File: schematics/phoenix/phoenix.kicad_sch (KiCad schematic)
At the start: 11 parts, among them U1 MAX31856, U2 NHD-C0220BIZ, U3 HHG1D-1

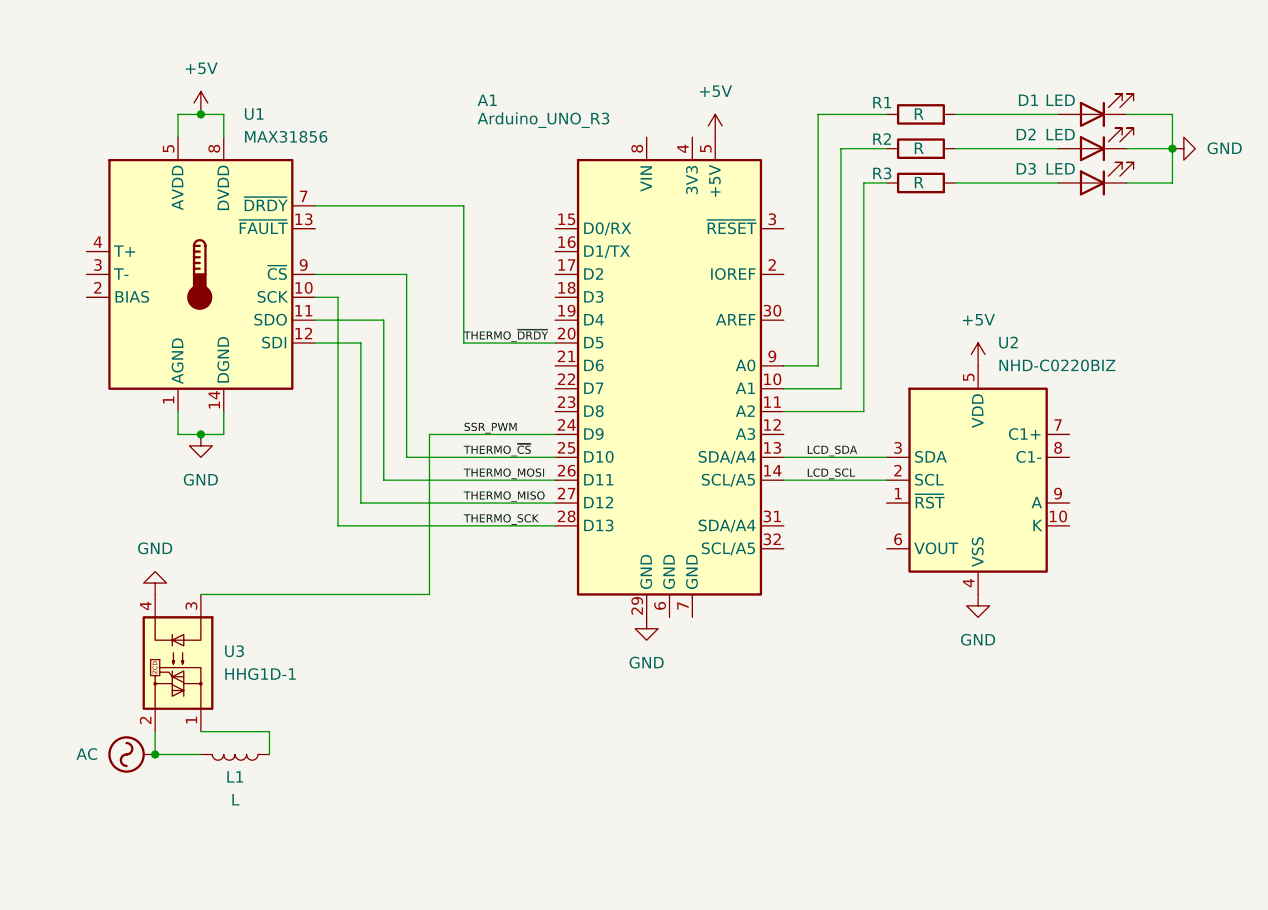
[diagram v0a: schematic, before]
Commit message: schematic done probably
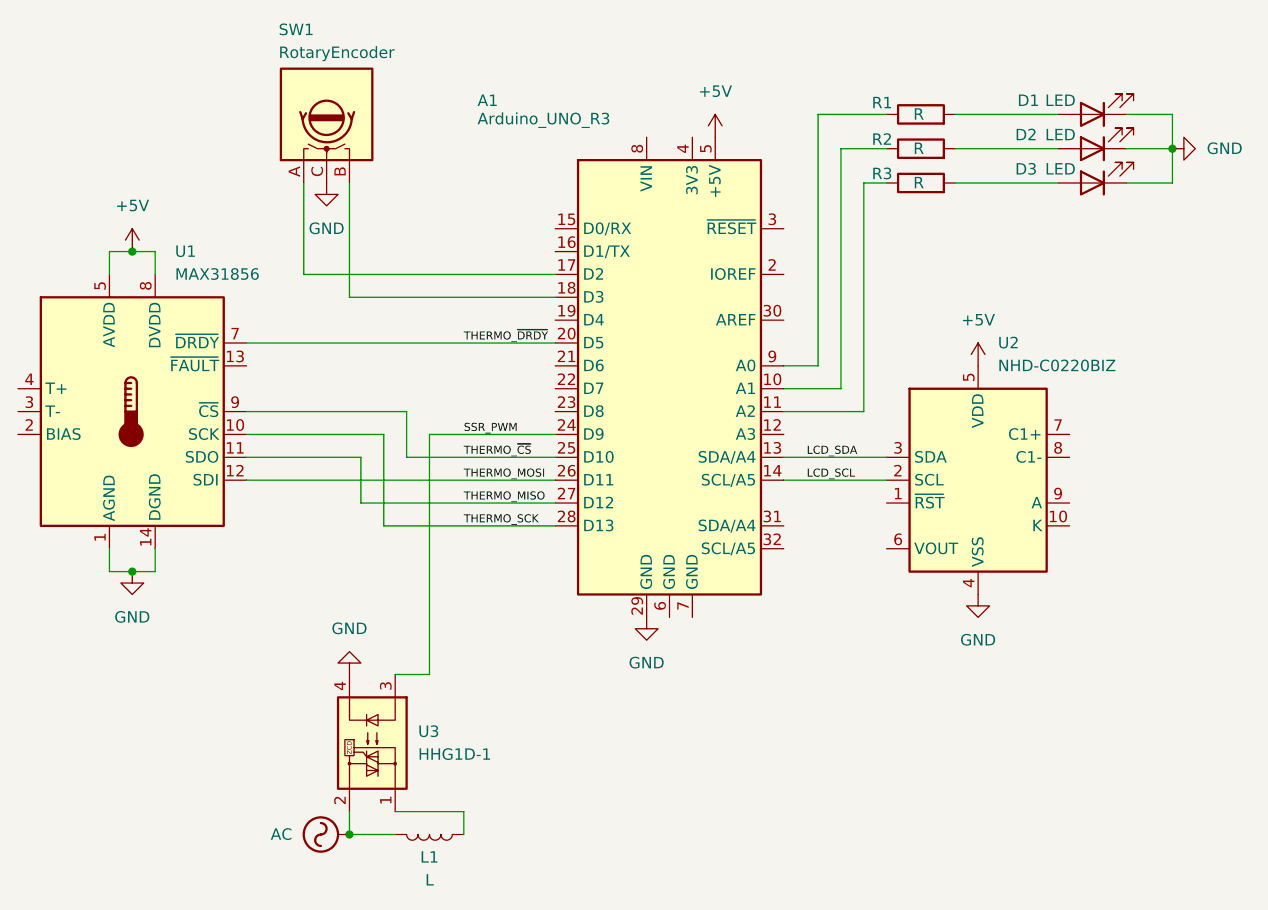
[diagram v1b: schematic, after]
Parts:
- added SW1: RotaryEncoder, symbol Device:RotaryEncoder
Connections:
- net GND: now also SW1.C
- net THERMO_MISO: now also U1.11 (SDO); no longer U1.12 (SDI)
- net THERMO_MOSI: now also U1.12 (SDI); no longer U1.11 (SDO)
- net at A1.17 (D2): now also SW1.A
- net at A1.18 (D3): now also SW1.B
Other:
- title: (none) -> Phoenix - Tube Furnace
- moved on the sheet: L1, U1, U3
